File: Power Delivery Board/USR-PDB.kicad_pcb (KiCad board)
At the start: 2 copper layers, 110 x 150 mm, 44 parts, among them IC1 LM7805ECT, IC2 LM7805ECT, J1 XT90PW-M, U10 Anderson PP45 Vert. 2x1, U11 Anderson PP45 Vert. 2x1, U12 Anderson PP45 Vert. 2x1, U14 MCP3002-I/P, U17 AMS1117-3.3, U2 Anderson PP45 Vert. 2x1, U3 Anderson PP45 Vert. 2x1, U4 Anderson PP45 Vert. 2x1, U5 Anderson PP45 Vert. 2x1, U6 Anderson PP45 Vert. 2x1, U7 LM2676T-12_NOPB

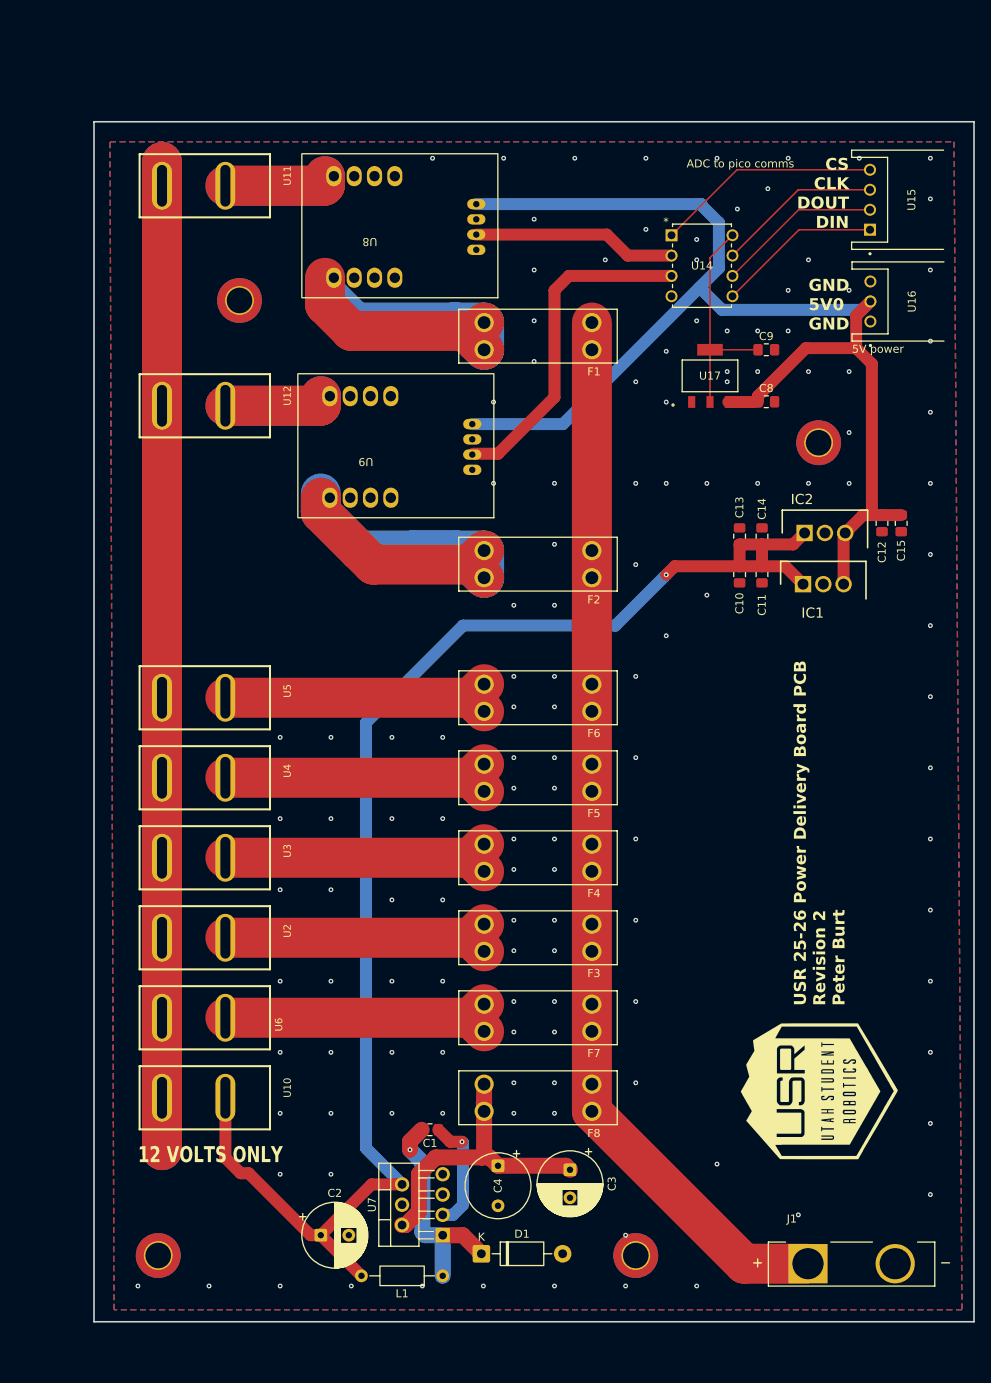
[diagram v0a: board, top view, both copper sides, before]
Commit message: Complete redesign of PDB pcb
AAAAAAAAAAAAAAAAAAAAAAAAAAAAAAAAAAAAAAAAAAAA
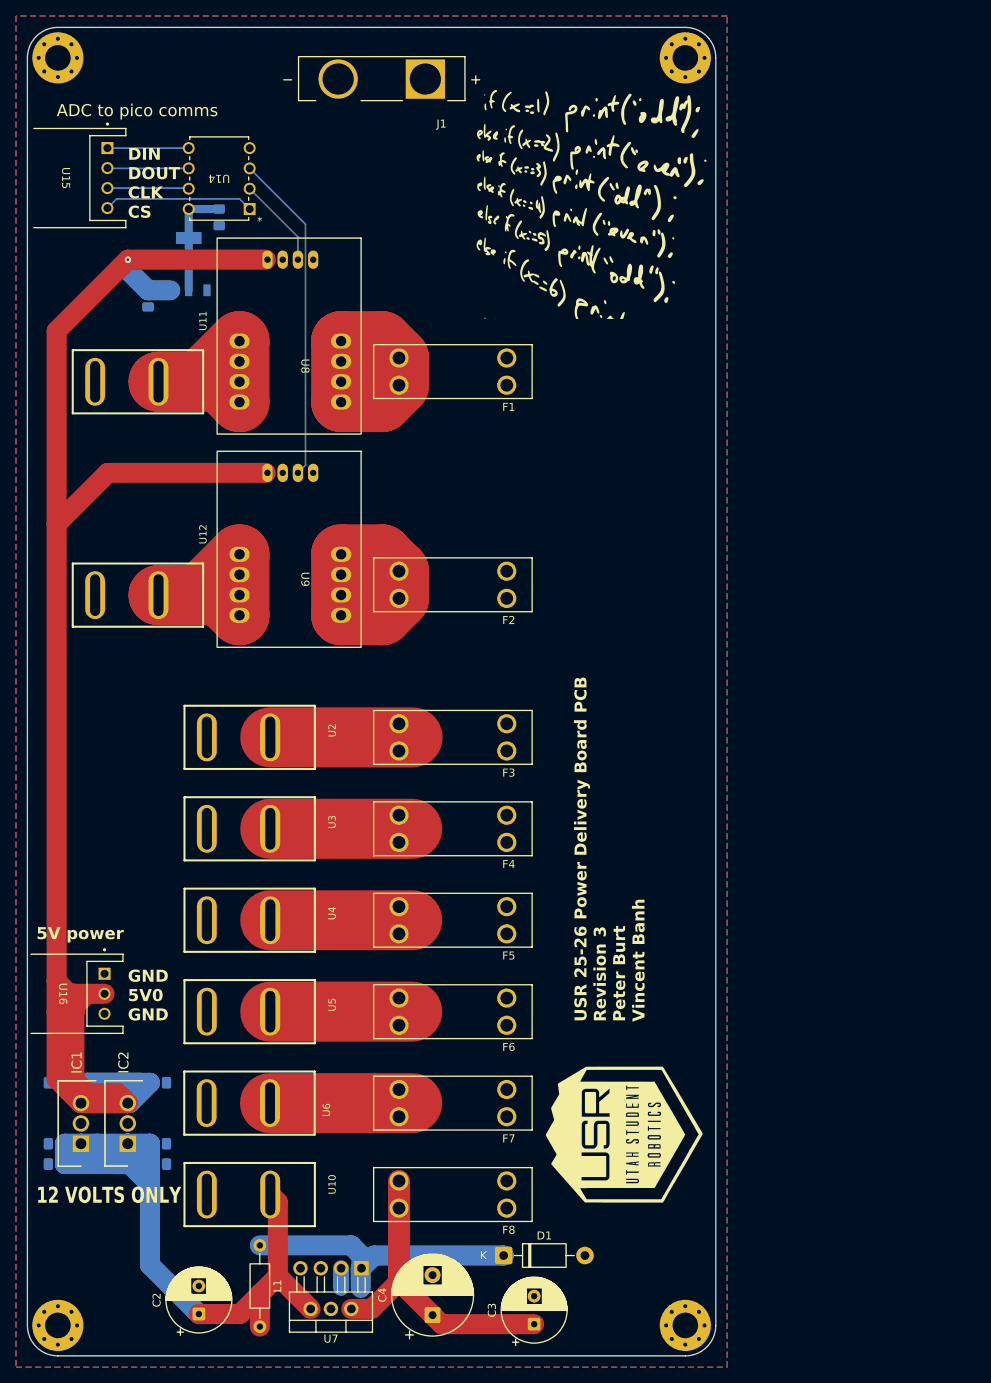
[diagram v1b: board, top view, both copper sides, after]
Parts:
- removed the REF** at (132.1, 71.1)
- removed the REF** at (59.7, 53.3)
- removed the REF** at (49.5, 172.7)
- removed the REF** at (109.2, 172.7)
- added G***: LOGO, LOGO, F.Cu at (104.1, 40.6)
- added REF**: MountingHole_3.2mm_M3_Pad_Via, MountingHole:MountingHole_3.2mm_M3_Pad_Via, F.Cu at (37.0, 23.0)
- added REF**: MountingHole_3.2mm_M3_Pad_Via, MountingHole:MountingHole_3.2mm_M3_Pad_Via, F.Cu at (115.4, 181.5)
- added REF**: MountingHole_3.2mm_M3_Pad_Via, MountingHole:MountingHole_3.2mm_M3_Pad_Via, F.Cu at (37.0, 181.5)
- added REF**: MountingHole_3.2mm_M3_Pad_Via, MountingHole:MountingHole_3.2mm_M3_Pad_Via, F.Cu at (115.4, 23.0)
- C1, C10, C11, C12, C13, C14, C15, C8, C9, U17: moved to B.Cu
- C4: footprint Capacitor_THT:CP_Radial_Tantal_D8.0mm_P5.00mm -> Capacitor_THT:CP_Radial_D10.0mm_P5.00mm
- moved J1 159.8 mm to (77.5, 25.4), turned to 180 degrees
- moved U16 137.7 mm to (37.1, 140.0), turned to -90 degrees
- moved C15 126.6 mm to (36.8, 151.1), turned to 180 degrees
- moved C14 118.0 mm to (36.8, 161.3), turned to 180 degrees
- moved C12 114.3 mm to (49.5, 151.1), turned to 0 degrees
- moved C13 114.3 mm to (36.8, 158.8), turned to 180 degrees
- moved IC1 114.2 mm to (39.9, 158.7), turned to 90 degrees
- moved IC2 114.0 mm to (45.7, 158.7), turned to 90 degrees
- moved U15 106.8 mm to (37.5, 38.0), turned to -90 degrees
- moved C11 103.7 mm to (49.5, 158.8), turned to 0 degrees
- moved C10 103.5 mm to (49.5, 161.3), turned to 0 degrees
- moved C8 78.3 mm to (48.3, 53.1), turned to -90 degrees
- moved C9 70.4 mm to (57.1, 42.9), turned to -90 degrees
- moved U17 66.6 mm to (53.3, 48.8), turned to 180 degrees
- moved U14 52.8 mm to (61.0, 41.9), turned to 180 degrees
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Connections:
- U8 pad 3: unconnected-(U8-in_2-Pad3) -> HE_sensor1
- U8 pad 4: unconnected-(U8-in_3-Pad4) -> HE_sensor1
- U8 pad 5: unconnected-(U8-in_4-Pad5) -> HE_sensor1
- U8 pad 6: unconnected-(U8-out_4-Pad6) -> Net-(U11-VCC)
- U8 pad 7: unconnected-(U8-out_3-Pad7) -> Net-(U11-VCC)
- U8 pad 8: unconnected-(U8-out_2-Pad8) -> Net-(U11-VCC)
- U9 pad 3: unconnected-(U9-in_2-Pad3) -> HE_sensor2
- U9 pad 4: unconnected-(U9-in_3-Pad4) -> HE_sensor2
- U9 pad 5: unconnected-(U9-in_4-Pad5) -> HE_sensor2
- U9 pad 6: unconnected-(U9-out_4-Pad6) -> Net-(U12-VCC)
- U9 pad 7: unconnected-(U9-out_3-Pad7) -> Net-(U12-VCC)
- U9 pad 8: unconnected-(U9-out_2-Pad8) -> Net-(U12-VCC)
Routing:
- net GND: track 247.0 -> 0.00 mm, vias 132 -> 0
- net Vin: track 133.3 -> 0.00 mm
- net 5V_OUT: track 160.8 -> 241.0 mm, vias 0 -> 1
- net 12V_OUT: track 180.8 -> 101.0 mm, vias 1 -> 0
- net HE_sensor2: track 66.6 -> 27.2 mm
- net HE_sensor1: track 59.5 -> 27.2 mm
- net Net-(U2-VCC): track 38.9 -> 17.8 mm
- net Net-(U5-VCC): track 35.9 -> 17.8 mm
- net Net-(U4-VCC): track 35.9 -> 17.8 mm
- net Net-(U3-VCC): track 35.5 -> 17.8 mm
- net Net-(U6-VCC): track 35.5 -> 17.8 mm
- net HE1_out: track 25.5 -> 11.4 mm
- net 3.3V_out: track 28.0 -> 14.0 mm
- net Net-(U7-BOOST): track 14.6 -> 2.45 mm, vias 1 -> 0
- net Din: track 20.6 -> 10.2 mm
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- added copper zone on F.Cu, net Vin
- removed copper zone on F.Cu, net GND
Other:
- board size 110 x 150 mm -> 86.1 x 166.1 mm
- board text added: "DIN DOUT CLK CS"
- board text added: "USR 25-26 Power Delivery Board PCB Revision 3 Peter Burt Vincent Banh"
- board text removed: "CS CLK DOUT DIN"
- board text removed: "USR 25-26 Power Delivery Board PCB Revision 2 Peter Burt"
